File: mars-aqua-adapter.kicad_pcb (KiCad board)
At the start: 2 copper layers, 35.7 x 37.2 mm, 38 parts, among them J1 Conn_01x03, J2 Conn_01x03, J3 Conn_01x04, J4 Conn_01x04, Q1 PNP, Q2 PNP, U1 LM358, U2 LM393

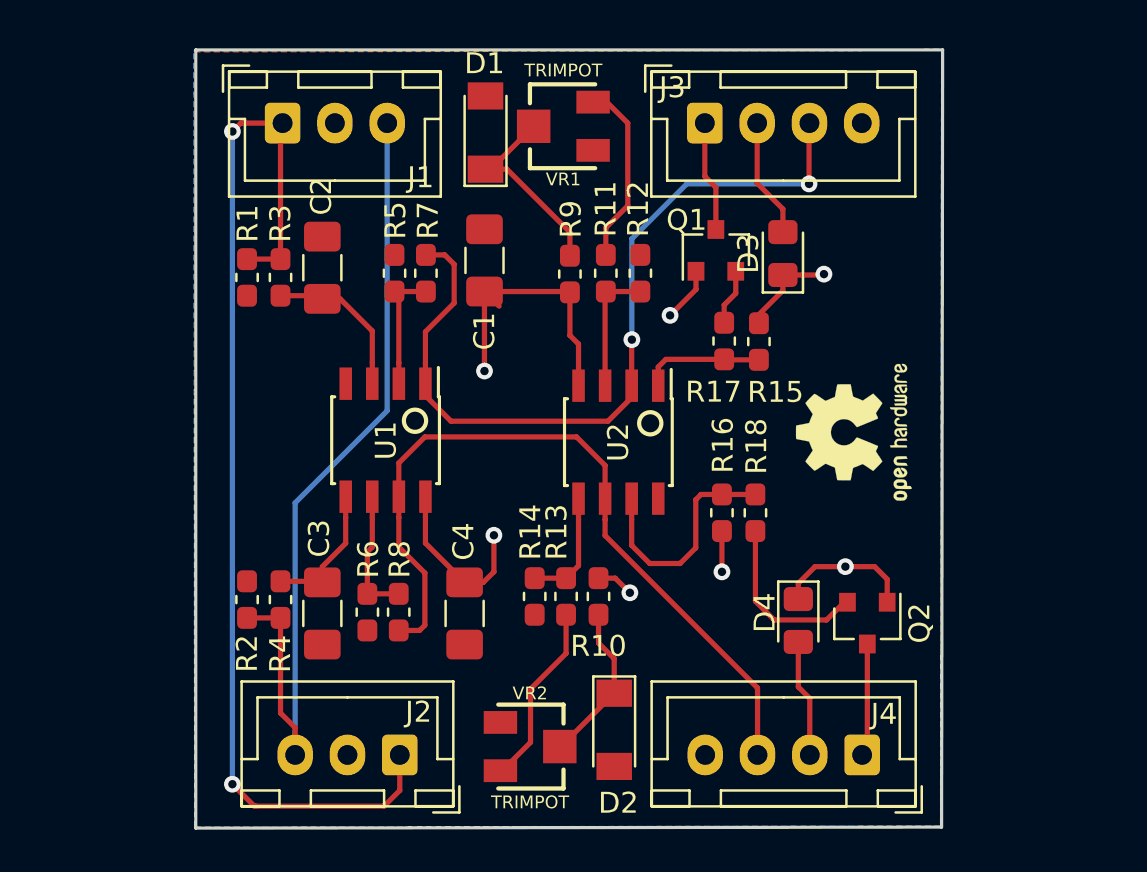
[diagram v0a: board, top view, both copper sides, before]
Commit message: board layout
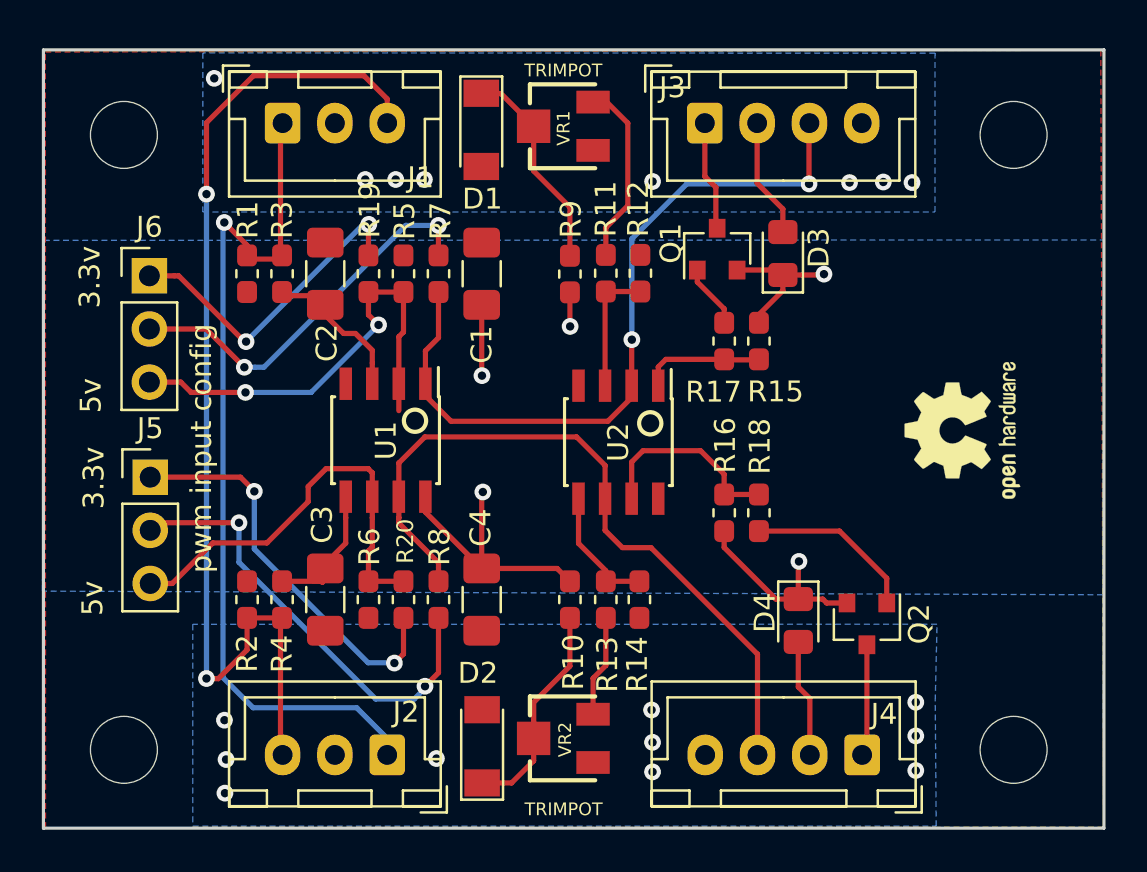
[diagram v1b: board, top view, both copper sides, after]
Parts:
- added J5: Conn_01x03, Connector_PinHeader_2.54mm:PinHeader_1x03_P2.54mm_Vertical, F.Cu at (111.9, 96.9)
- added J6: Conn_01x03, Connector_PinHeader_2.54mm:PinHeader_1x03_P2.54mm_Vertical, F.Cu at (111.8, 87.3)
- added R19: 100k, Resistor_SMD:R_0603_1608Metric_Pad1.05x0.95mm_HandSolder, F.Cu at (122.3, 87.2)
- added R20: 100k, Resistor_SMD:R_0603_1608Metric_Pad1.05x0.95mm_HandSolder, F.Cu at (124.0, 102.8)
- added REF**: MountingHole_3.2mm_M3, MountingHole:MountingHole_3.2mm_M3, F.Cu at (110.6, 80.6)
- added REF**: MountingHole_3.2mm_M3, MountingHole:MountingHole_3.2mm_M3, F.Cu at (110.6, 110.0)
- added REF**: MountingHole_3.2mm_M3, MountingHole:MountingHole_3.2mm_M3, F.Cu at (153.1, 110.0)
- added REF**: MountingHole_3.2mm_M3, MountingHole:MountingHole_3.2mm_M3, F.Cu at (153.1, 80.6)
- Q1, Q2: value PNP -> Q_PNP_BEC
- R7, R8: value 330k -> 100k
- moved D2 6.36 mm to (127.7, 109.8), turned to 90 degrees
- moved REF** 5.19 mm to (150.7, 94.7)
- moved R14 5.01 mm to (135.3, 102.8)
- moved R8 1.99 mm to (125.7, 102.8)
- moved R13 1.91 mm to (133.7, 102.8)
- moved VR2 1.64 mm to (131.6, 109.4), turned to 90 degrees
- moved R10 1.38 mm to (131.9, 102.8)
- moved C4 1.05 mm to (127.7, 102.8)
- moved C3 0.68 mm to (120.2, 102.8)
- moved C1 0.65 mm to (127.7, 87.2)
- moved R7 0.60 mm to (125.7, 87.2)
- moved R6 0.60 mm to (122.3, 102.8)
- moved J2 0.60 mm to (123.2, 110.2)
- moved R5 0.43 mm to (124.0, 87.2)
- moved C2 0.32 mm to (120.2, 87.2)
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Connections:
- Q1 pad 1: +12V -> Net-(Q1-Pad1)
- Q1 pad 2: Net-(Q1-Pad2) -> +12V
- Q2 pad 1: +12V -> Net-(Q2-Pad1)
- Q2 pad 2: Net-(Q2-Pad2) -> +12V
- R17 pad 1: Net-(Q1-Pad2) -> Net-(Q1-Pad1)
- R18 pad 1: Net-(Q2-Pad2) -> Net-(Q2-Pad1)
- R5 pad 1: Net-(R5-Pad1) -> Net-(J6-Pad3)
- R6 pad 1: Net-(R6-Pad1) -> Net-(J5-Pad3)
- R7 pad 1: /ch1_output -> Net-(J6-Pad2)
- R7 pad 2: Net-(R5-Pad1) -> /ch1_output
- R8 pad 1: /ch2_output -> Net-(J5-Pad2)
- R8 pad 2: Net-(R6-Pad1) -> /ch2_output
- U1 pad 2: Net-(R5-Pad1) -> Net-(J6-Pad3)
- U1 pad 6: Net-(R6-Pad1) -> Net-(J5-Pad3)
- U2 pad 4: +12V -> (no net)
- U2 pad 8: GND -> (no net)
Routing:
- net Net-(J6-Pad3): track 0.00 -> 22.7 mm, vias 0 -> 2
- net Net-(J5-Pad2): track 0.00 -> 21.7 mm, vias 0 -> 2
- net Net-(J5-Pad3): track 0.00 -> 20.3 mm
- net Net-(J5-Pad1): track 0.00 -> 19.3 mm, vias 0 -> 2
- net Net-(J6-Pad2): track 0.00 -> 18.8 mm, vias 0 -> 2
- net Net-(J6-Pad1): track 0.00 -> 15.6 mm, vias 0 -> 2
- net /ch1_input: track 52.4 -> 42.0 mm, vias 2 -> 1
- net /ch2_input: track 40.5 -> 50.0 mm, vias 0 -> 2
- net Net-(Q2-Pad2): track 8.47 -> 0.00 mm
- net Net-(Q2-Pad1): track 0.00 -> 8.23 mm
- net Net-(R5-Pad1): track 6.42 -> 0.00 mm
- net Net-(R6-Pad1): track 6.24 -> 0.00 mm
- net +12V: track 39.6 -> 35.1 mm, vias 7 -> 5
- net Net-(R13-Pad1): track 8.80 -> 4.86 mm
- net /ch1_output: track 38.7 -> 35.0 mm
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- added copper zone on B.Cu, net GND
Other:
- board size 35.7 x 37.2 mm -> 50.7 x 37.2 mm
- board text added: "3.3v"
- board text added: "5v"
- board text added: "pwm input config"
